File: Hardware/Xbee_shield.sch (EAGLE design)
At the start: 38 parts, among them Q1 MOSFET-NCHANNELSMD, Q2 MOSFET-NCHANNELSMD, U1 ARDUINO_SHIELD, U2 XBEE-1B3, U4 V_REG_LDOSMD

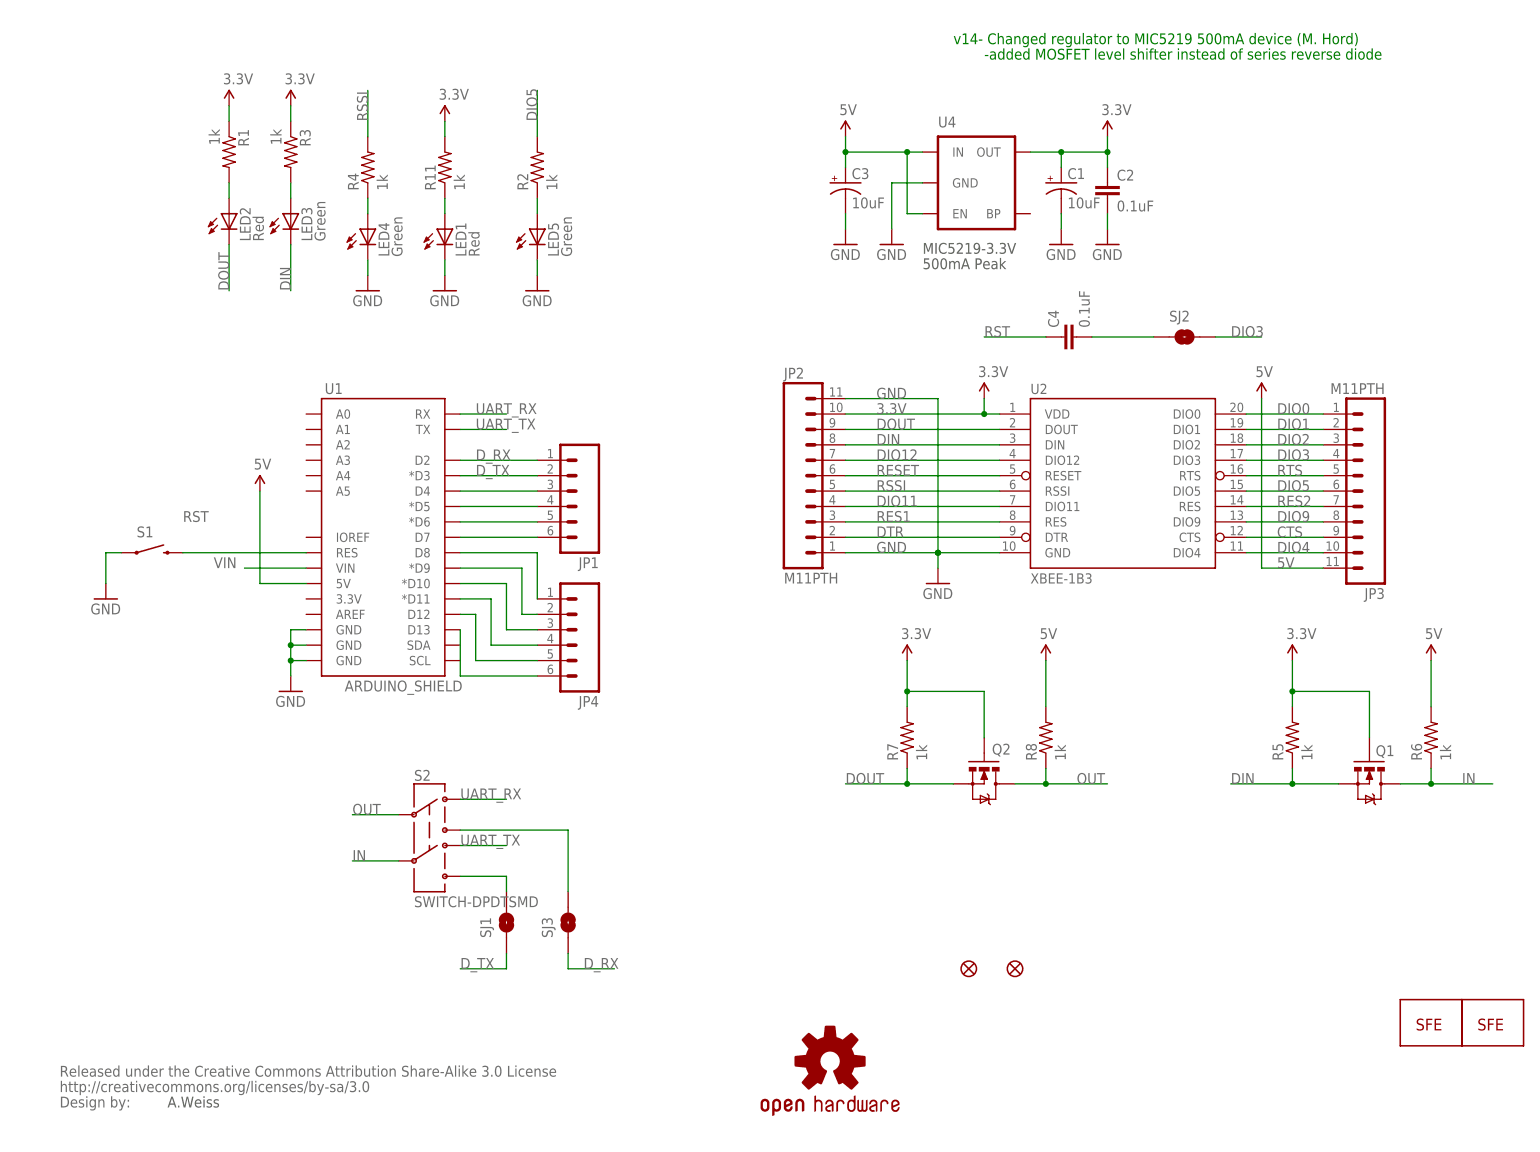
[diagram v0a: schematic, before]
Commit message: Sch work
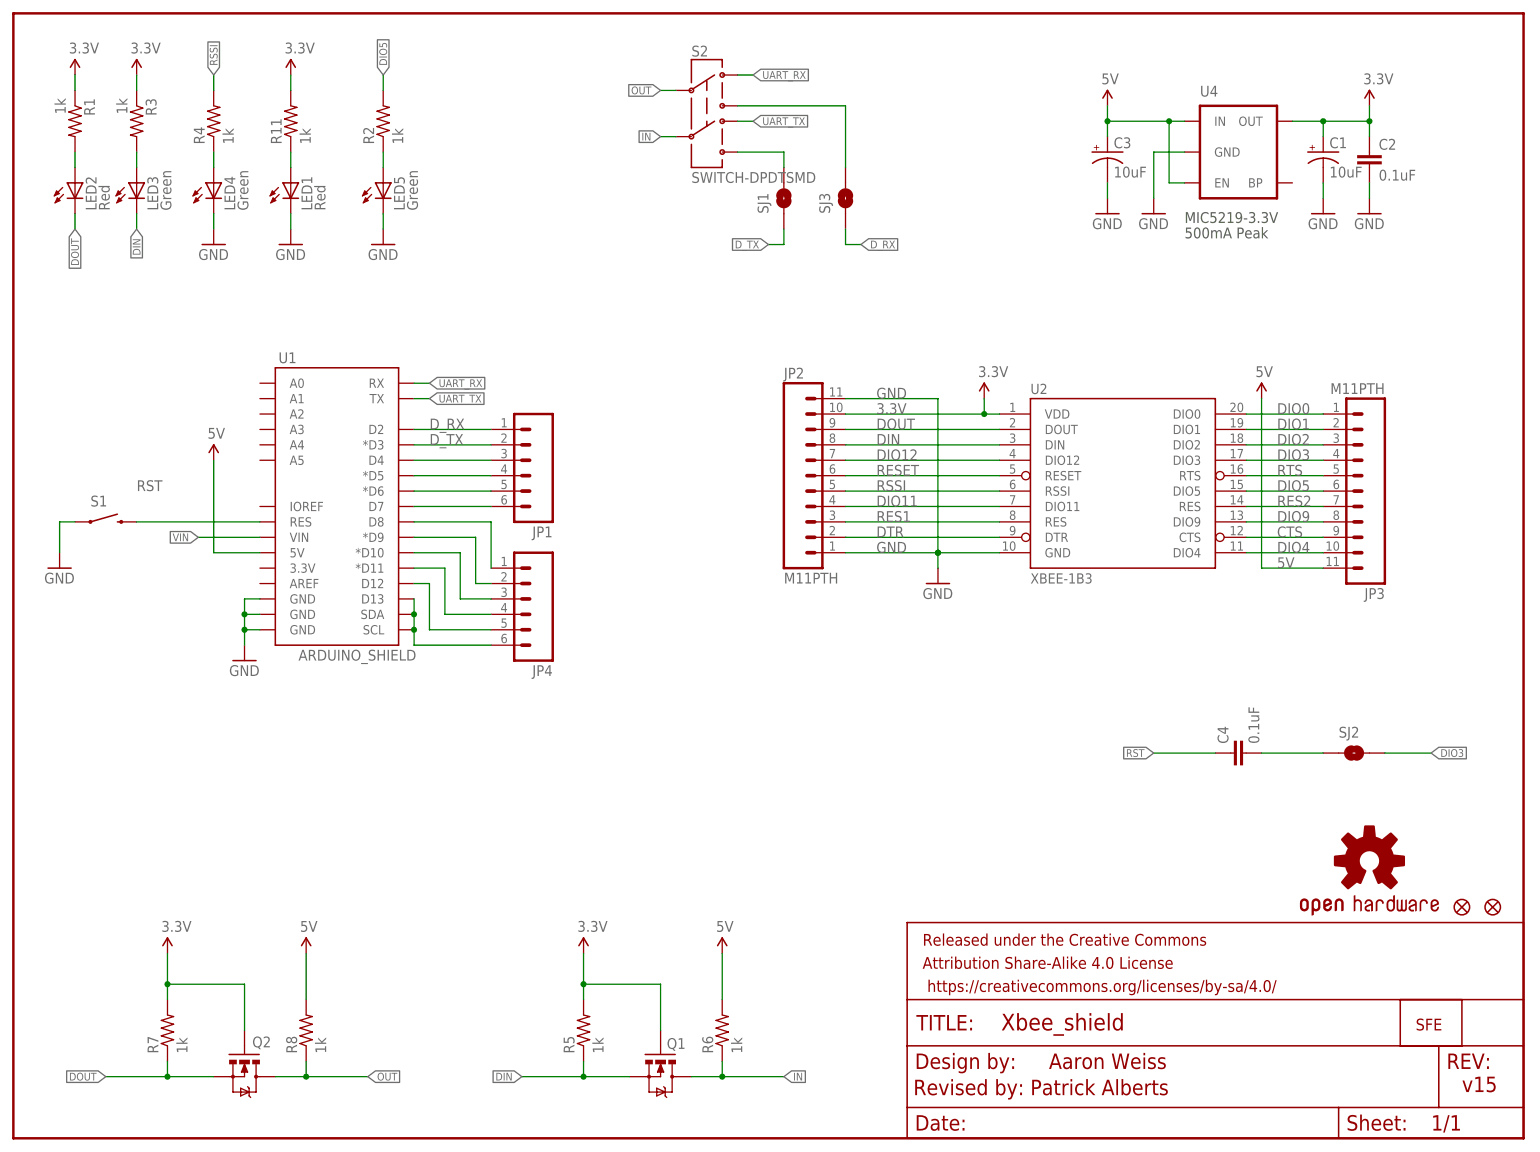
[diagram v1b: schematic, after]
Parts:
- removed U$1: LOGO-SFESK, SparkFun:LOGO-SFESK
- removed U$5: CREATIVE_COMMONS, SparkFun:CREATIVE_COMMONS
- added FRAME1: FRAME-LETTER, SparkFun-Aesthetics:FRAME-LETTER
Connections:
- net N$67: now also U1.SCL, U1.SDA
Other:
- note added: "Aaron Weiss"
- note added: "Revised by: Patrick Alberts"
- note added: "v15"
- note removed: "-added MOSFET level shifter instead of series reverse diode"
- note removed: "A.Weiss"
- note removed: "v14- Changed regulator to MIC5219 500mA device (M. Hord)"
- moved on the sheet: C1, C2, C3, C4, JP1, JP4, LED1, LED2, LED3, LED4, LED5, Q1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
